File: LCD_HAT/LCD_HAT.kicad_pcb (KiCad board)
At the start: 2 copper layers, 45.7 x 53.3 mm, 8 parts, among them J2 LCD

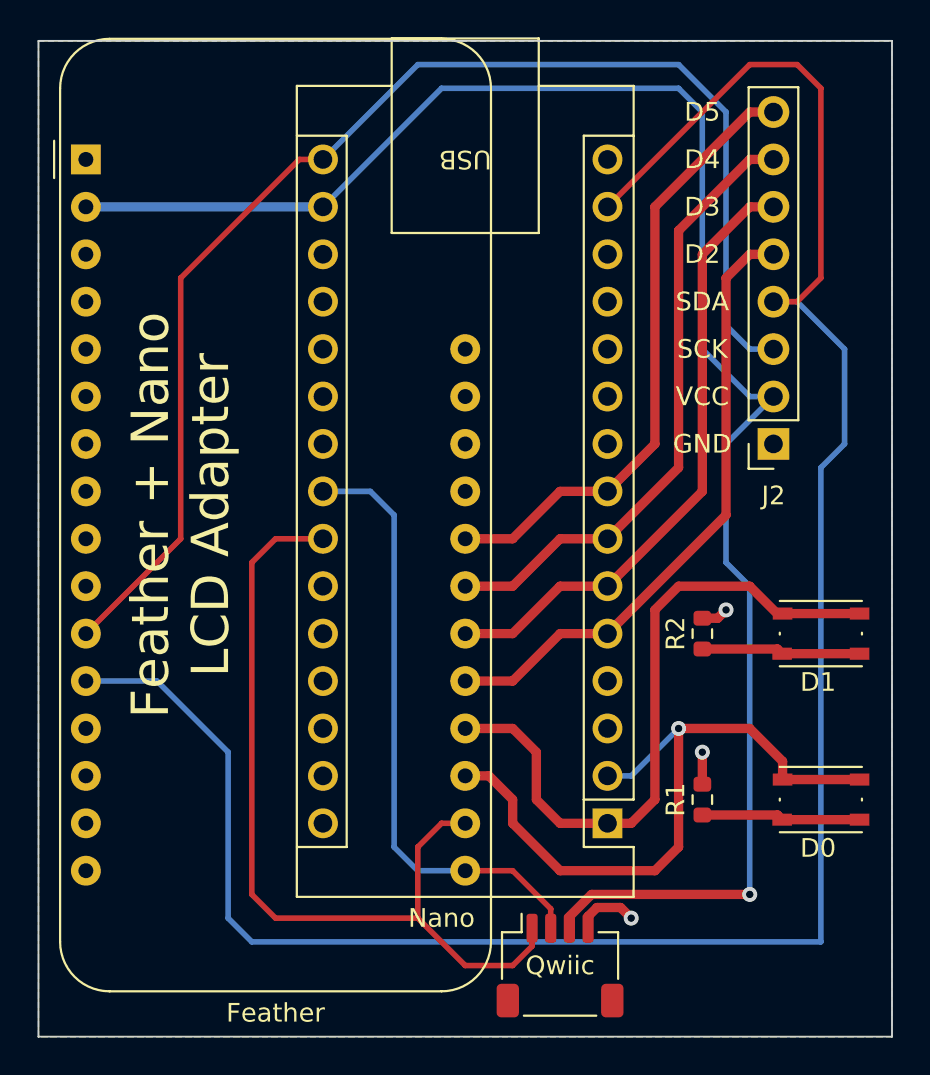
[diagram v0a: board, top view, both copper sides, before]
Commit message: Updated project files
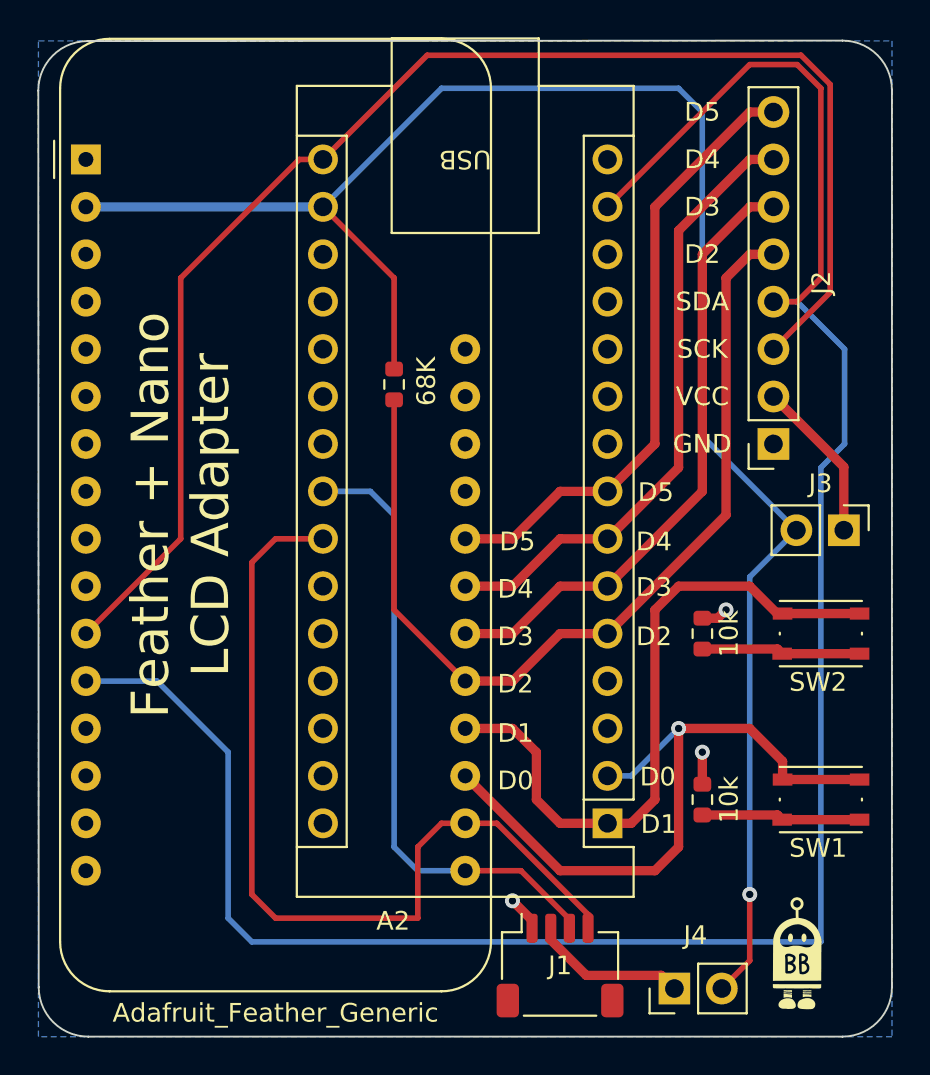
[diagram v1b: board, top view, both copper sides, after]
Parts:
- added G***: LOGO, LOGO, F.Cu at (152.4, 114.9)
- added J3: PWR_JUMPER, Connector_PinHeader_2.54mm:PinHeader_1x02_P2.54mm_Vertical, F.Cu at (154.9, 92.2)
- added J4: PWR_JUMPER, Connector_PinHeader_2.54mm:PinHeader_1x02_P2.54mm_Vertical, F.Cu at (145.8, 116.8)
- added R3: 68K, Resistor_SMD:R_0603_1608Metric, F.Cu at (130.8, 84.4)
- A1: value Feather -> Adafruit_Feather_Generic
- renumbered Nano to A2, Qwiic to J1, D0 to SW1, D1 to SW2
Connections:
- A1 pad 17: Net-(A1-Pad17) -> Net-(A1-SDA)
- A1 pad 18: Net-(A1-Pad18) -> Net-(A1-SCL)
- A2 pad 23: Net-(A1-Pad17) -> Net-(A1-SDA)
- A2 pad 24: Net-(A1-Pad18) -> Net-(A1-SCL)
- J1 pad 1: Net-(A1-Pad18) -> GND
- J1 pad 2: Net-(A1-Pad17) -> Net-(J1-Pin_2)
- J1 pad 3: +3.3V -> Net-(A1-SDA)
- J1 pad 4: GND -> Net-(A1-SCL)
- J2 pad 2: +3.3V -> Net-(J2-Pin_2)
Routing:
- net Net-(A1-SCL): track 0.00 -> 48.4 mm
- net Net-(A1-Pad18): track 47.0 -> 0.00 mm
- net Net-(A1-SDA): track 0.00 -> 33.6 mm
- net Net-(A1-Pad17): track 32.9 -> 0.00 mm
- net Net-(A1-D2): track 33.4 -> 50.1 mm
- net Net-(J2-Pin_2): track 0.00 -> 8.72 mm
- net Net-(J1-Pin_2): track 0.00 -> 8.33 mm
- net Net-(A1-SCK): track 70.6 -> 77.0 mm
- net +3.3V: track 92.8 -> 97.1 mm
- net GND: track 6.55 -> 5.07 mm
- net Net-(A1-D0): track 37.4 -> 36.7 mm
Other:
- board size 45.7 x 53.3 mm -> 45.7 x 53.4 mm
- board text added: "D0"
- board text added: "D1"
